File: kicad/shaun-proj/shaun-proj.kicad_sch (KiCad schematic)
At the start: 41 parts, among them J1 USB_C_Receptacle_PowerOnly_6P, J2 Conn_02x16_Odd_Even, J3 Conn_01x02_Socket, Q1 AO3401A, Q2 AO3400A, Q4 AO3400A, Q5 AO3400A, SW1 SW_SPDT, SW2 SW_SPDT, U1 CH224K, U3 INA219AxD, U4 XL1509-5.0, U5 TP4056-42-ESOP8

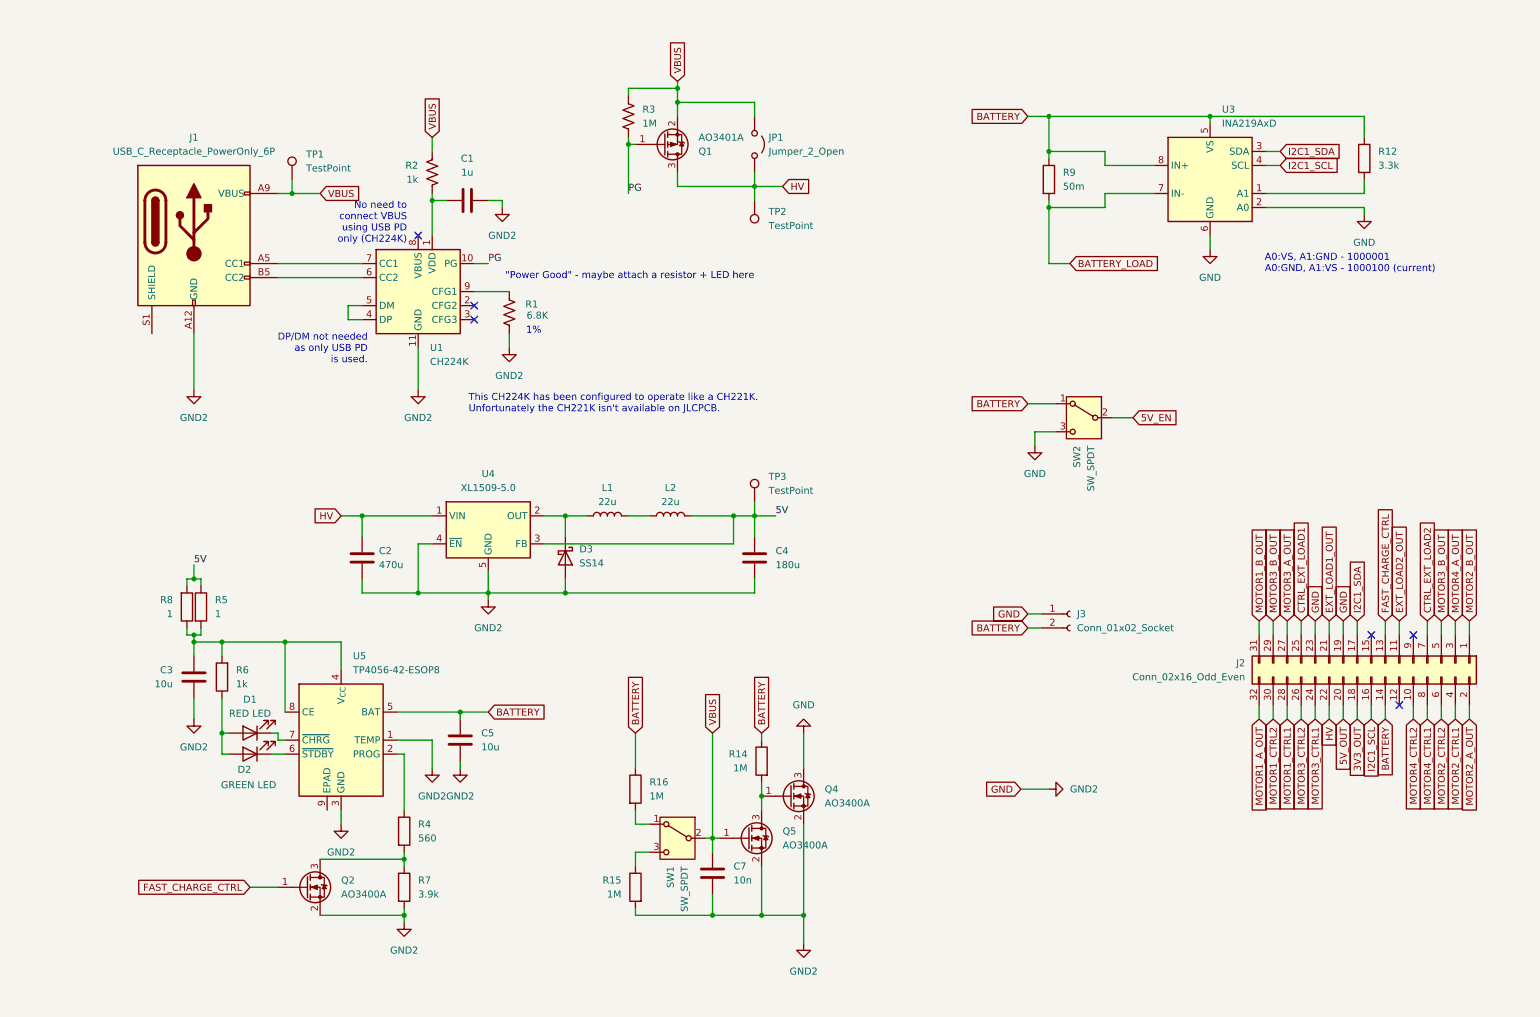
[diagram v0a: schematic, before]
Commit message: switching, improvements, PCB start
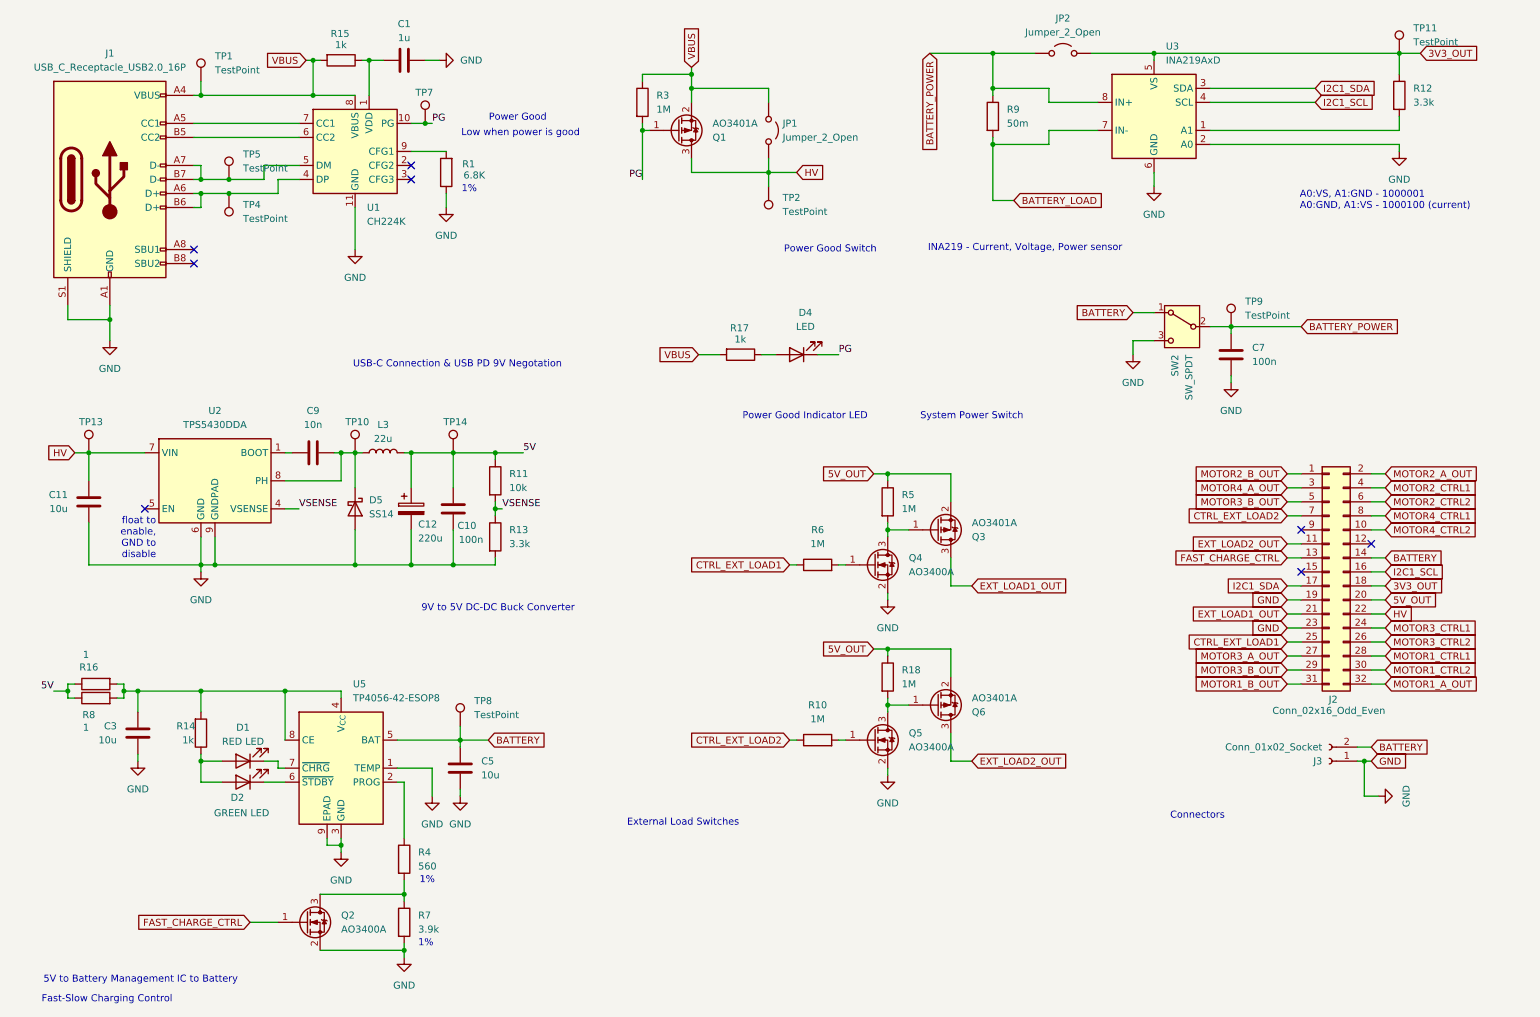
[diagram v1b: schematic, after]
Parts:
- removed C2: 470u, symbol Device:C
- removed C4: 180u, symbol Device:C
- removed D3: SS14, Diode_SMD:D_SMA, symbol Diode:SS14
- removed J1: USB_C_Receptacle_PowerOnly_6P, Connector_USB:USB_C_Receptacle_HRO_TYPE-C-31-M-17, symbol Connector:USB_C_Receptacle_PowerOnly_6P
- removed L1: 22u, Inductor_SMD:L_SXN_SMDRI125, symbol Device:L
- removed L2: 22u, symbol Device:L
- removed R2: 1k, symbol Device:R_US
- removed SW1: SW_SPDT, symbol Switch:SW_SPDT
- removed TP3: TestPoint, TestPoint:TestPoint_Pad_D1.5mm, symbol Connector:TestPoint
- removed U4: XL1509-5.0, Package_SO:SOIC-8_3.9x4.9mm_P1.27mm, symbol Regulator_Switching:XL1509-5.0
- added C10: 100n, Capacitor_SMD:C_0603_1608Metric_Pad1.08x0.95mm_HandSolder, symbol Device:C
- added C11: 10u, Capacitor_SMD:C_0805_2012Metric_Pad1.18x1.45mm_HandSolder, symbol Device:C
- added C12: 220u, Capacitor_SMD:CP_Elec_6.3x7.7, symbol Device:C_Polarized
- added C9: 10n, Capacitor_SMD:C_0402_1005Metric_Pad0.74x0.62mm_HandSolder, symbol Device:C
- added D4: LED, LED_SMD:LED_0805_2012Metric_Pad1.15x1.40mm_HandSolder, symbol Device:LED
- added D5: SS14, Diode_SMD:D_SMA, symbol Diode:SS14
- added J1: USB_C_Receptacle_USB2.0_16P, MyLibrary:USB_C_Receptacle_G-Switch_GT-USB-7010ASV_MOD, symbol Connector:USB_C_Receptacle_USB2.0_16P
- added JP2: Jumper_2_Open, TestPoint:TestPoint_2Pads_Pitch2.54mm_Drill0.8mm, symbol Jumper:Jumper_2_Open
- added L3: 22u, Inductor_SMD:L_SXN_SMDRI125, symbol Device:L
- added Q3, Q6: AO3401A, Package_TO_SOT_SMD:SOT-23, symbol Transistor_FET:AO3401A
- added R10, R18: 1M, Resistor_SMD:R_0603_1608Metric, symbol Device:R
- added R11: 10k, Resistor_SMD:R_0603_1608Metric_Pad0.98x0.95mm_HandSolder, symbol Device:R
- added R13: 3.3k, Resistor_SMD:R_0603_1608Metric_Pad0.98x0.95mm_HandSolder, symbol Device:R
- added R17: 1k, Resistor_SMD:R_0603_1608Metric_Pad0.98x0.95mm_HandSolder, symbol Device:R
- added TP10, TP11, TP13, TP14, TP4, TP5, TP7, TP8, TP9: TestPoint, TestPoint:TestPoint_Pad_D1.5mm, symbol Connector:TestPoint
- added U2: TPS5430DDA, Package_SO:SOIC-8-1EP_3.9x4.9mm_P1.27mm_EP2.514x3.2mm, symbol Regulator_Switching:TPS5430DDA
- C1: footprint (none) -> Capacitor_SMD:C_0402_1005Metric_Pad0.74x0.62mm_HandSolder; JLC (none) -> https://jlcpcb.com/partdetail/53938-CL05A105KA5NQNC/C52923
- C3: footprint (none) -> Capacitor_SMD:C_0603_1608Metric_Pad1.08x0.95mm_HandSolder
- C5: footprint (none) -> Capacitor_SMD:C_0603_1608Metric_Pad1.08x0.95mm_HandSolder; LCSC (none) -> C19702
- C7: value 10n -> 100n; footprint (none) -> Capacitor_SMD:C_0603_1608Metric_Pad1.08x0.95mm_HandSolder
- D1: footprint (none) -> LED_SMD:LED_0603_1608Metric_Pad1.05x0.95mm_HandSolder
- D2: footprint (none) -> LED_SMD:LED_0805_2012Metric_Pad1.15x1.40mm_HandSolder
- J2: footprint (none) -> Connector_PinHeader_2.54mm:PinHeader_2x16_P2.54mm_Vertical
- Q4, Q5: LCSC (none) -> C20917
- R1, R3: symbol Device:R_US -> Device:R
- R12: footprint Resistor_SMD:R_0603_1608Metric -> Resistor_SMD:R_0603_1608Metric_Pad0.98x0.95mm_HandSolder
- R14: value 1M -> 1k; footprint (none) -> Resistor_SMD:R_0603_1608Metric_Pad0.98x0.95mm_HandSolder; JLC (none) -> https://jlcpcb.com/partdetail/21904-0603WAF1001T5E/C21190
- R15: value 1M -> 1k; footprint (none) -> Resistor_SMD:R_0603_1608Metric_Pad0.98x0.95mm_HandSolder; JLC (none) -> https://jlcpcb.com/partdetail/21904-0603WAF1001T5E/C21190; LSCS (none) -> C21190
- R16: value 1M -> 1; footprint (none) -> Resistor_SMD:R_0805_2012Metric_Pad1.20x1.40mm_HandSolder; JLC (none) -> https://jlcpcb.com/partdetail/26014-0805W8F100KT5E/C25271
- R5: value 1 -> 1M; footprint (none) -> Resistor_SMD:R_0603_1608Metric
- R6: value 1k -> 1M
- R8: footprint (none) -> Resistor_SMD:R_0805_2012Metric_Pad1.20x1.40mm_HandSolder; JLC (none) -> https://jlcpcb.com/partdetail/26014-0805W8F100KT5E/C25271
- SW2: footprint (none) -> MyLibrary:SS-12D11G3R
- U1: LCSC (none) -> C970725
- U5: footprint Package_SO:SOIC-8-1EP_3.9x4.9mm_P1.27mm_EP2.41x3.3mm_ThermalVias -> Package_SO:SOIC-8-1EP_3.9x4.9mm_P1.27mm_EP2.41x3.3mm; LCSC (none) -> C9864
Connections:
- net 3V3_OUT: now also R12.1, U3.5 (VS), JP2.2 (B), TP11.1
- net 5V: now also R16.1, R8.1, C10.1, C12.1, L3.2, R11.1, TP14.1; no longer R5.1, R8.2
- net 5V_OUT: now also R5.1, Q3.2 (S), Q6.2 (S), R18.1
- net BATTERY: now also TP8.1; no longer R12.1, R14.1, R16.1, R9.1, U3.5 (VS), U3.8 (IN+)
- net CTRL_EXT_LOAD1: now also R6.1
- net CTRL_EXT_LOAD2: now also R10.1
- net EXT_LOAD1_OUT: now also Q3.3 (D)
- net EXT_LOAD2_OUT: now also Q6.3 (D)
- net GND: now also U5.9 (EPAD), C10.2, C11.2, C12.2, D5.2 (A), J1.A1 (GND), J1.A12 (GND), J1.B1 (GND), J1.B12 (GND), J1.S1 (SHIELD), R13.2, U2.6 (GND), U2.9 (GNDPAD); no longer Q4.3 (D), R15.2
- net HV: now also C11.1, TP13.1, U2.7 (VIN)
- net PG: now also D4.1 (K), TP7.1
- net VBUS: now also R15.2, U1.8 (VBUS), J1.A4 (VBUS), J1.A9 (VBUS), J1.B4 (VBUS), J1.B9 (VBUS), R17.2; no longer C7.1, Q5.1 (G)
- net at C1.1, U1.1 (VDD): now also R15.1
- net at C3.1, U5.4 (V_{CC}), U5.8 (CE): now also R14.2, R16.2, R8.2; no longer R5.2, R6.2, R8.1
- net at U1.5 (DM): now also J1.A7 (D-), J1.B7 (D-), TP5.1; no longer U1.4 (DP)
- net at U1.6 (CC2): now also J1.B5 (CC2)
- net at U1.7 (CC1): now also J1.A5 (CC1)
- net at D1.2 (A), D2.2 (A): now also R14.1; no longer R6.1
- net 5V_EN renamed BATTERY_POWER
- net BATTERY_POWER: now also C7.1, R9.1, U3.8 (IN+), JP2.1 (A), TP9.1
- new net: Q5.3 (D), Q6.1 (G), R18.2
- new net: C9.2, D5.1 (K), L3.1, TP10.1, U2.8 (PH)
- new net: Q3.1 (G), Q4.3 (D), R5.2
- new net: J1.A6 (D+), J1.B6 (D+), TP4.1, U1.4 (DP)
- new net: Q5.1 (G), R10.2
- new net: C9.1, U2.1 (BOOT)
- new net: Q4.1 (G), R6.2
- new net: D4.2 (A), R17.1
- new net VSENSE: R11.2, R13.1, U2.4 (VSENSE)
- no-connect marks 6 -> 8
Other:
- note added: "5V to Battery Management IC to Battery"
- note added: "9V to 5V DC-DC Buck Converter"
- note added: "Connectors"
- note added: "External Load Switches"
- note added: "Fast-Slow Charging Control"
- note added: "INA219 - Current, Voltage, Power sensor"
- note added: "Low when power is good"
- note added: "Power Good"
- note added: "Power Good Indicator LED"
- note added: "Power Good Switch"
- note added: "System Power Switch"
- note added: "USB-C Connection & USB PD 9V Negotation"
- note added: "float to enable, GND to disable"
- note removed: ""Power Good" - maybe attach a resistor + LED here"
- note removed: "DP/DM not needed as only USB PD is used."
- note removed: "No need to connect VBUS using USB PD only (CH224K)"
- note removed: "This CH224K has been configured to operate like a CH221K. Unfortunately the CH221K isn't available on JLCPCB."
- title: (none) -> Micromouse Power Board
- moved on the sheet: C1, C3, C5, D1, D2, J2, J3, JP1, Q1, Q2, R12, R4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
